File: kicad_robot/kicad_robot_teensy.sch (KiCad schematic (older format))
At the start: 2 parts, among them U12->5 R-78E5.0-1.0

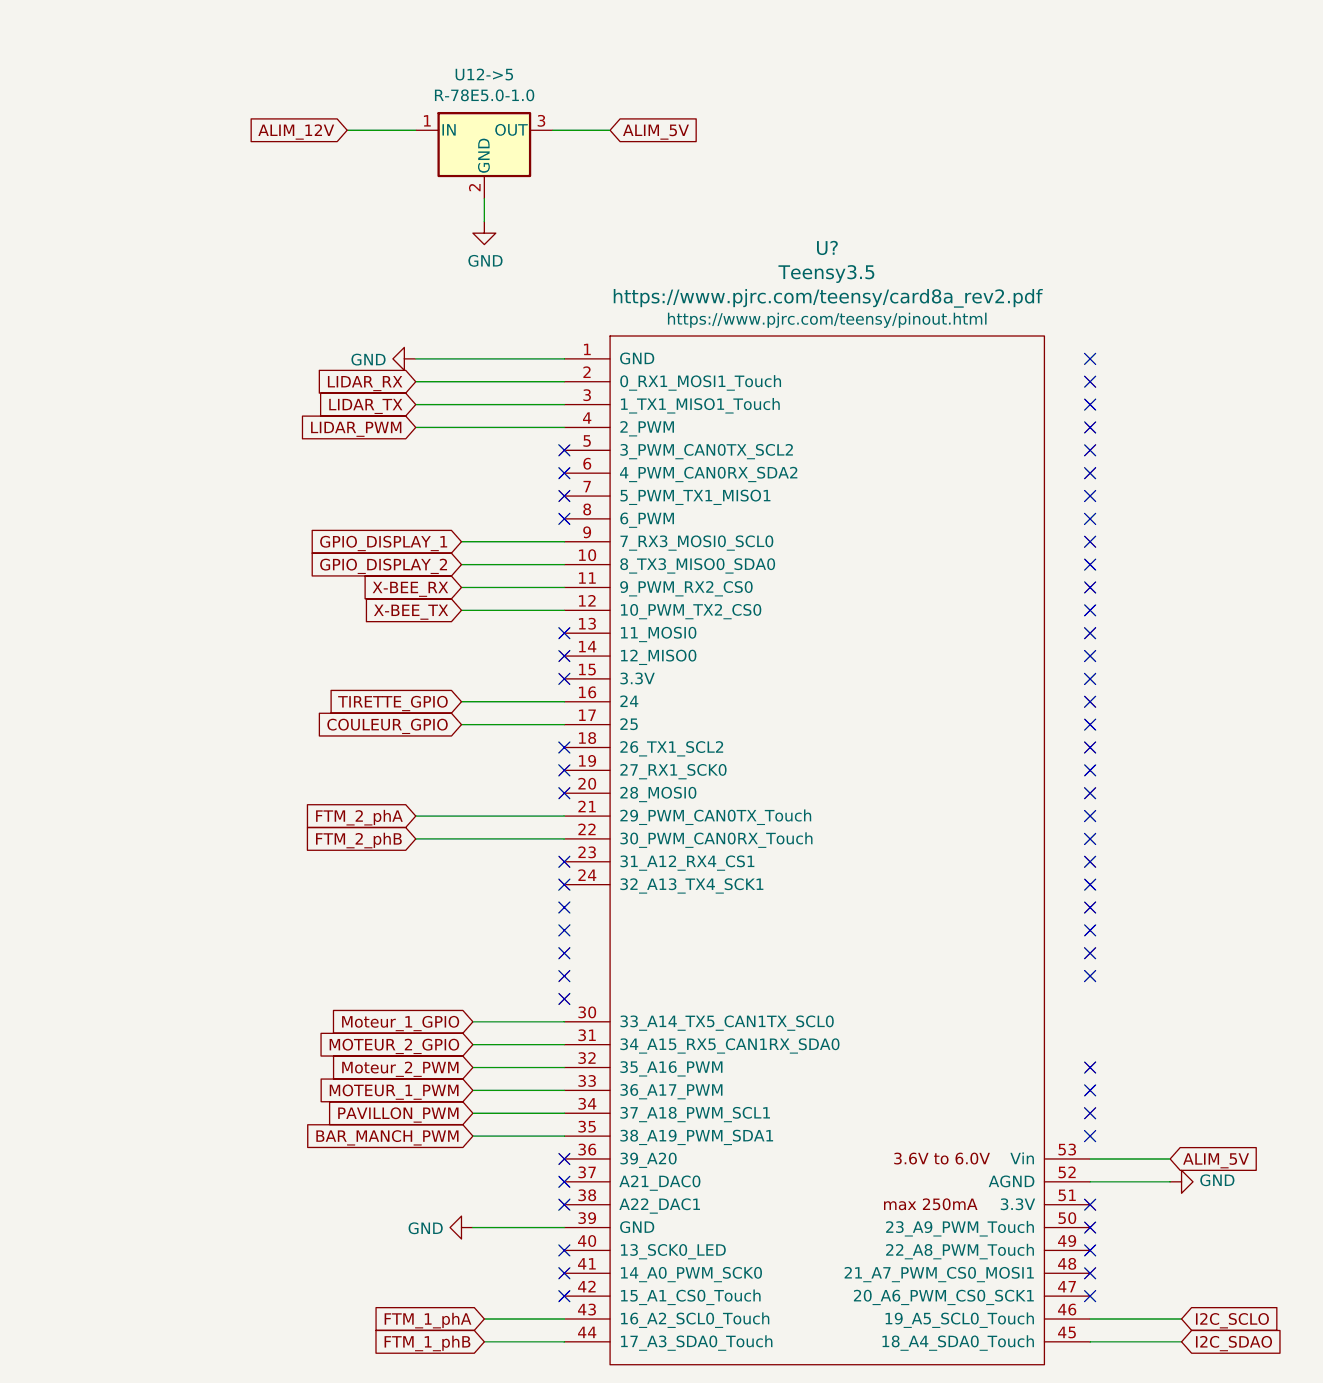
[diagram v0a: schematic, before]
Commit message: mise à jour
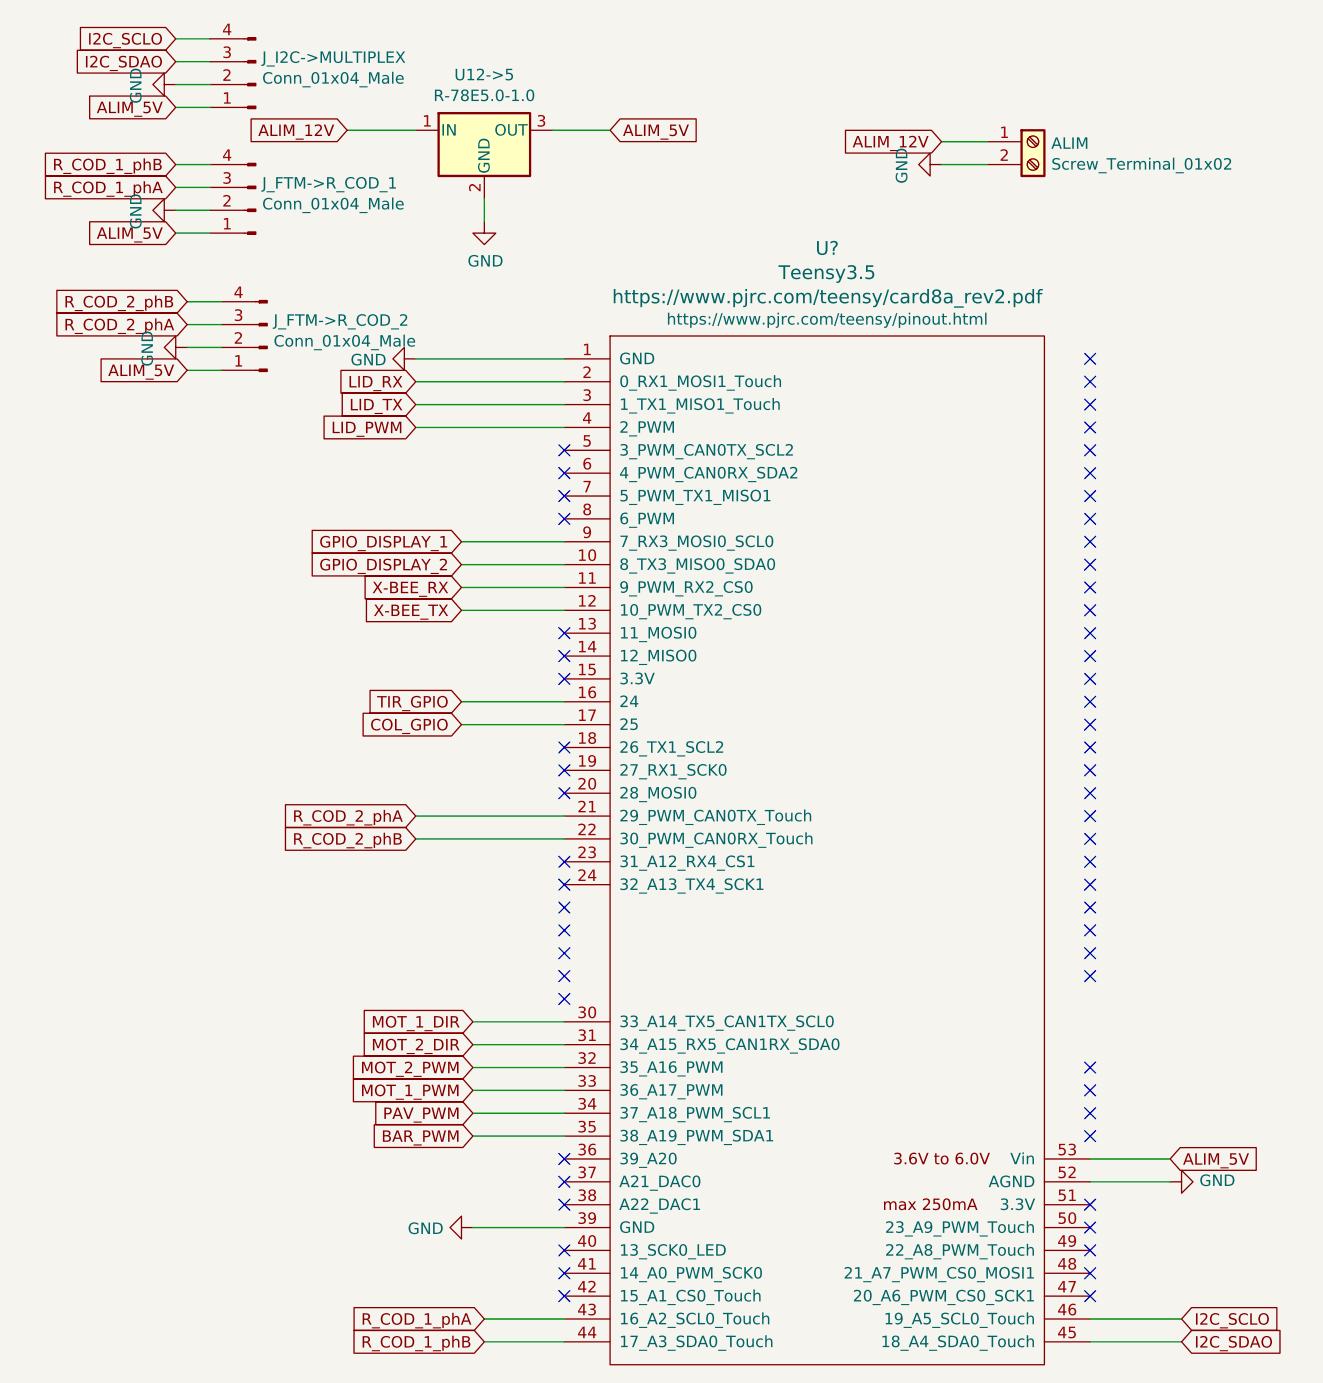
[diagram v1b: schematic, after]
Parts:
- added ALIM: Screw_Terminal_01x02, symbol Connector:Screw_Terminal_01x02
- added J_FTM->R_COD_1, J_FTM->R_COD_2, J_I2C->MULTIPLEX: Conn_01x04_Male, symbol Connector:Conn_01x04_Male
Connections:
- net ALIM_12V: now also ALIM.1 (Pin_1)
- net ALIM_5V: now also J_FTM->R_COD_1.1 (Pin_1), J_FTM->R_COD_2.1 (Pin_1), J_I2C->MULTIPLEX.1 (Pin_1)
- net GND: now also ALIM.2 (Pin_2), J_FTM->R_COD_1.2 (Pin_2), J_FTM->R_COD_2.2 (Pin_2), J_I2C->MULTIPLEX.2 (Pin_2)
- net I2C_SCLO: now also J_I2C->MULTIPLEX.4 (Pin_4)
- net I2C_SDAO: now also J_I2C->MULTIPLEX.3 (Pin_3)
- net BAR_MANCH_PWM renamed BAR_PWM
- net COULEUR_GPIO renamed COL_GPIO
- net FTM_1_phA renamed R_COD_1_phA
- net R_COD_1_phA: now also J_FTM->R_COD_1.3 (Pin_3)
- net FTM_1_phB renamed R_COD_1_phB
- net R_COD_1_phB: now also J_FTM->R_COD_1.4 (Pin_4)
- net FTM_2_phA renamed R_COD_2_phA
- net R_COD_2_phA: now also J_FTM->R_COD_2.3 (Pin_3)
- net FTM_2_phB renamed R_COD_2_phB
- net R_COD_2_phB: now also J_FTM->R_COD_2.4 (Pin_4)
- net LIDAR_PWM renamed LID_PWM
- net LIDAR_RX renamed LID_RX
- net LIDAR_TX renamed LID_TX
- net MOTEUR_1_PWM renamed MOT_1_PWM
- net MOTEUR_2_GPIO renamed MOT_2_DIR
- net Moteur_1_GPIO renamed MOT_1_DIR
- net Moteur_2_PWM renamed MOT_2_PWM
- net PAVILLON_PWM renamed PAV_PWM
- net TIRETTE_GPIO renamed TIR_GPIO
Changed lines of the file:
@@
 $EndComp
 Text GLabel 7450 2100 0    50   Input ~ 0
-LIDAR_RX
+LID_RX
 Text GLabel 7450 2200 0    50   Input ~ 0
-LIDAR_TX
+LID_TX
 Text GLabel 7450 2300 0    50   Input ~ 0
-LIDAR_PWM
+LID_PWM
 Text GLabel 7650 2800 0    50   Input ~ 0
 GPIO_DISPLAY_1
@@
 X-BEE_TX
 Text GLabel 7650 3500 0    50   Input ~ 0
-TIRETTE_GPIO
+TIR_GPIO
 $Comp
 L power:GND #PWR?
@@
 	10750 5500 10400 5500
 Text GLabel 7650 3600 0    50   Input ~ 0
-COULEUR_GPIO
+COL_GPIO
 Text GLabel 7450 4000 0    50   Input ~ 0
-FTM_2_phA
+R_COD_2_phA
 Text GLabel 7450 4100 0    50   Input ~ 0
-FTM_2_phB
+R_COD_2_phB
 Text GLabel 7700 4900 0    50   Input ~ 0
-Moteur_1_GPIO
+MOT_1_DIR
 Text GLabel 7700 5000 0    50   Input ~ 0
-MOTEUR_2_GPIO
+MOT_2_DIR
 Text GLabel 7700 5100 0    50   Input ~ 0
-Moteur_2_PWM
+MOT_2_PWM
 Text GLabel 7700 5200 0    50   Input ~ 0
-MOTEUR_1_PWM
+MOT_1_PWM
 Text GLabel 7700 5300 0    50   Input ~ 0
-PAVILLON_PWM
+PAV_PWM
 Text GLabel 7700 5400 0    50   Input ~ 0
-BAR_MANCH_PWM
+BAR_PWM
 Text GLabel 7750 6200 0    50   Input ~ 0
-FTM_1_phA
+R_COD_1_phA
 Text GLabel 7750 6300 0    50   Input ~ 0
-FTM_1_phB
+R_COD_1_phB
 Wire Wire Line
 	7750 6300 8100 6300
@@
 Wire Wire Line
 	7150 1000 7450 1000
+$Comp
+L Connector:Screw_Terminal_01x02 ALIM
+U 1 1 60342002
+P 10150 1050
+F 0 "ALIM" H 10230 1042 50  0000 L CNN
+F 1 "Screw_Terminal_01x02" H 10230 951 50  0000 L CNN
+F 2 "" H 10150 1050 50  0001 C CNN
+F 3 "~" H 10150 1050 50  0001 C CNN
+	1    10150 1050
+	1    0    0    -1
+$EndComp
+Text GLabel 9750 1050 0    50   Input ~ 0
+ALIM_12V
+$Comp
+L power:GND #PWR?
+U 1 1 60342E59
+P 9750 1150
+F 0 "#PWR?" H 9750 900 50  0001 C CNN
+F 1 "GND" H 9755 977 50  0000 C CNN
+F 2 "" H 9750 1150 50  0001 C CNN
+F 3 "" H 9750 1150 50  0001 C CNN
+	1    9750 1150
+	0    1    1    0
+$EndComp
+Wire Wire Line
+	9750 1150 9950 1150
+Wire Wire Line
+	9750 1050 9950 1050
+$Comp
+L Connector:Conn_01x04_Male J_I2C->MULTIPLEX
+U 1 1 60344D96
+P 6750 800
+F 0 "J_I2C->MULTIPLEX" H 6722 682 50  0000 R CNN
+F 1 "Conn_01x04_Male" H 6722 773 50  0000 R CNN
+F 2 "" H 6750 800 50  0001 C CNN
+F 3 "~" H 6750 800 50  0001 C CNN
+	1    6750 800
+	-1   0    0    1
+$EndComp
+$Comp
+L power:GND #PWR?
+U 1 1 6034965D
+P 6400 800
+F 0 "#PWR?" H 6400 550 50  0001 C CNN
+F 1 "GND" H 6405 627 50  0000 C CNN
+F 2 "" H 6400 800 50  0001 C CNN
+F 3 "" H 6400 800 50  0001 C CNN
+	1    6400 800
+	0    1    1    0
+$EndComp
+Text GLabel 6400 900  0    50   Input ~ 0
+ALIM_5V
+Text GLabel 6400 700  0    50   Input ~ 0
+I2C_SDAO
+Text GLabel 6400 600  0    50   Input ~ 0
+I2C_SCLO
+Wire Wire Line
+	6400 600  6550 600
+Wire Wire Line
+	6400 700  6550 700
+Wire Wire Line
+	6400 800  6550 800
+Wire Wire Line
+	6400 900  6550 900
+$Comp
+L Connector:Conn_01x04_Male J_FTM->R_COD_1
+U 1 1 6034C8A3
+P 6750 1350
+F 0 "J_FTM->R_COD_1" H 6722 1232 50  0000 R CNN
+F 1 "Conn_01x04_Male" H 6722 1323 50  0000 R CNN
+F 2 "" H 6750 1350 50  0001 C CNN
+F 3 "~" H 6750 1350 50  0001 C CNN
+	1    6750 1350
+	-1   0    0    1
+$EndComp
+Text GLabel 6400 1450 0    50   Input ~ 0
+ALIM_5V
+$Comp
+L power:GND #PWR?
+U 1 1 6034D5A6
+P 6400 1350
+F 0 "#PWR?" H 6400 1100 50  0001 C CNN
+F 1 "GND" H 6405 1177 50  0000 C CNN
+F 2 "" H 6400 1350 50  0001 C CNN
+F 3 "" H 6400 1350 50  0001 C CNN
+	1    6400 1350
+	0    1    1    0
+$EndComp
+Text GLabel 6400 1250 0    50   Input ~ 0
+R_COD_1_phA
+Text GLabel 6400 1150 0    50   Input ~ 0
+R_COD_1_phB
+Wire Wire Line
+	6400 1150 6550 1150
+Wire Wire Line
+	6550 1250 6400 1250
+Wire Wire Line
+	6400 1350 6550 1350
+Wire Wire Line
+	6550 1450 6400 1450
+$Comp
+L Connector:Conn_01x04_Male J_FTM->R_COD_2
+U 1 1 6035325F
+P 6800 1950
+F 0 "J_FTM->R_COD_2" H 6772 1832 50  0000 R CNN
+F 1 "Conn_01x04_Male" H 6772 1923 50  0000 R CNN
+F 2 "" H 6800 1950 50  0001 C CNN
+F 3 "~" H 6800 1950 50  0001 C CNN
+	1    6800 1950
+	-1   0    0    1
+$EndComp
+Text GLabel 6450 2050 0    50   Input ~ 0
+ALIM_5V
+$Comp
+L power:GND #PWR?
+U 1 1 60353D5D
+P 6450 1950
+F 0 "#PWR?" H 6450 1700 50  0001 C CNN
+F 1 "GND" H 6455 1777 50  0000 C CNN
+F 2 "" H 6450 1950 50  0001 C CNN
+F 3 "" H 6450 1950 50  0001 C CNN
+	1    6450 1950
+	0    1    1    0
+$EndComp
+Text GLabel 6450 1850 0    50   Input ~ 0
+R_COD_2_phA
+Text GLabel 6450 1750 0    50   Input ~ 0
+R_COD_2_phB
+Wire Wire Line
+	6450 1750 6600 1750
+Wire Wire Line
+	6600 1850 6450 1850
+Wire Wire Line
+	6450 1950 6600 1950
+Wire Wire Line
+	6600 2050 6450 2050
 $EndSCHEMATC

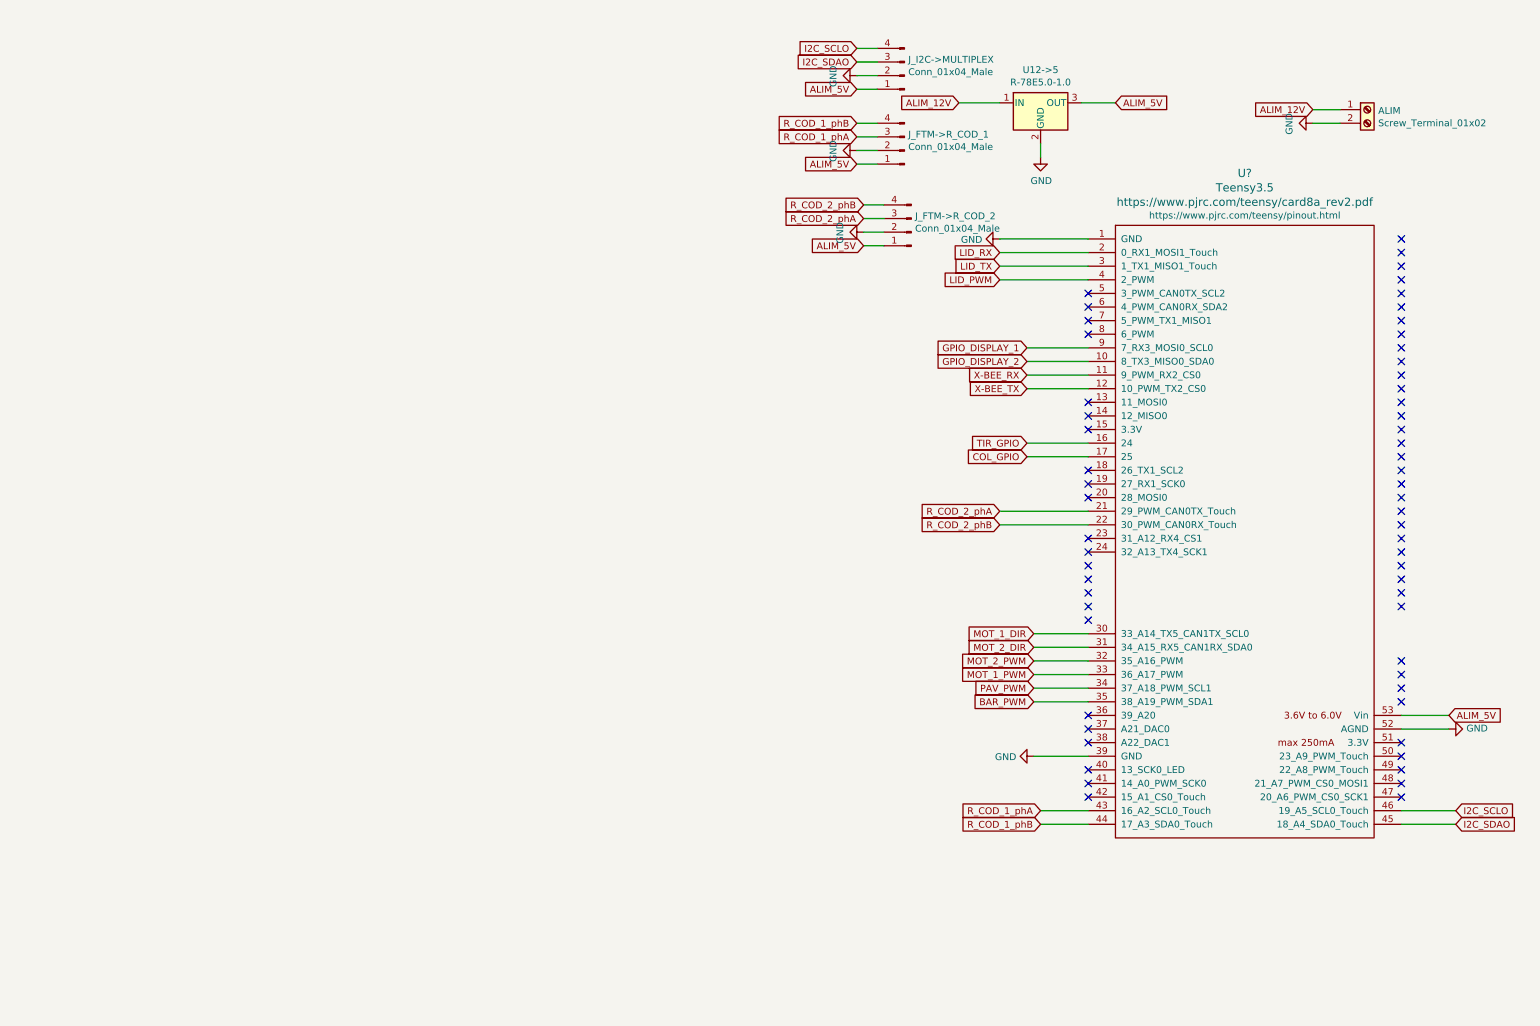
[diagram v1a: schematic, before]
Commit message: MAJ
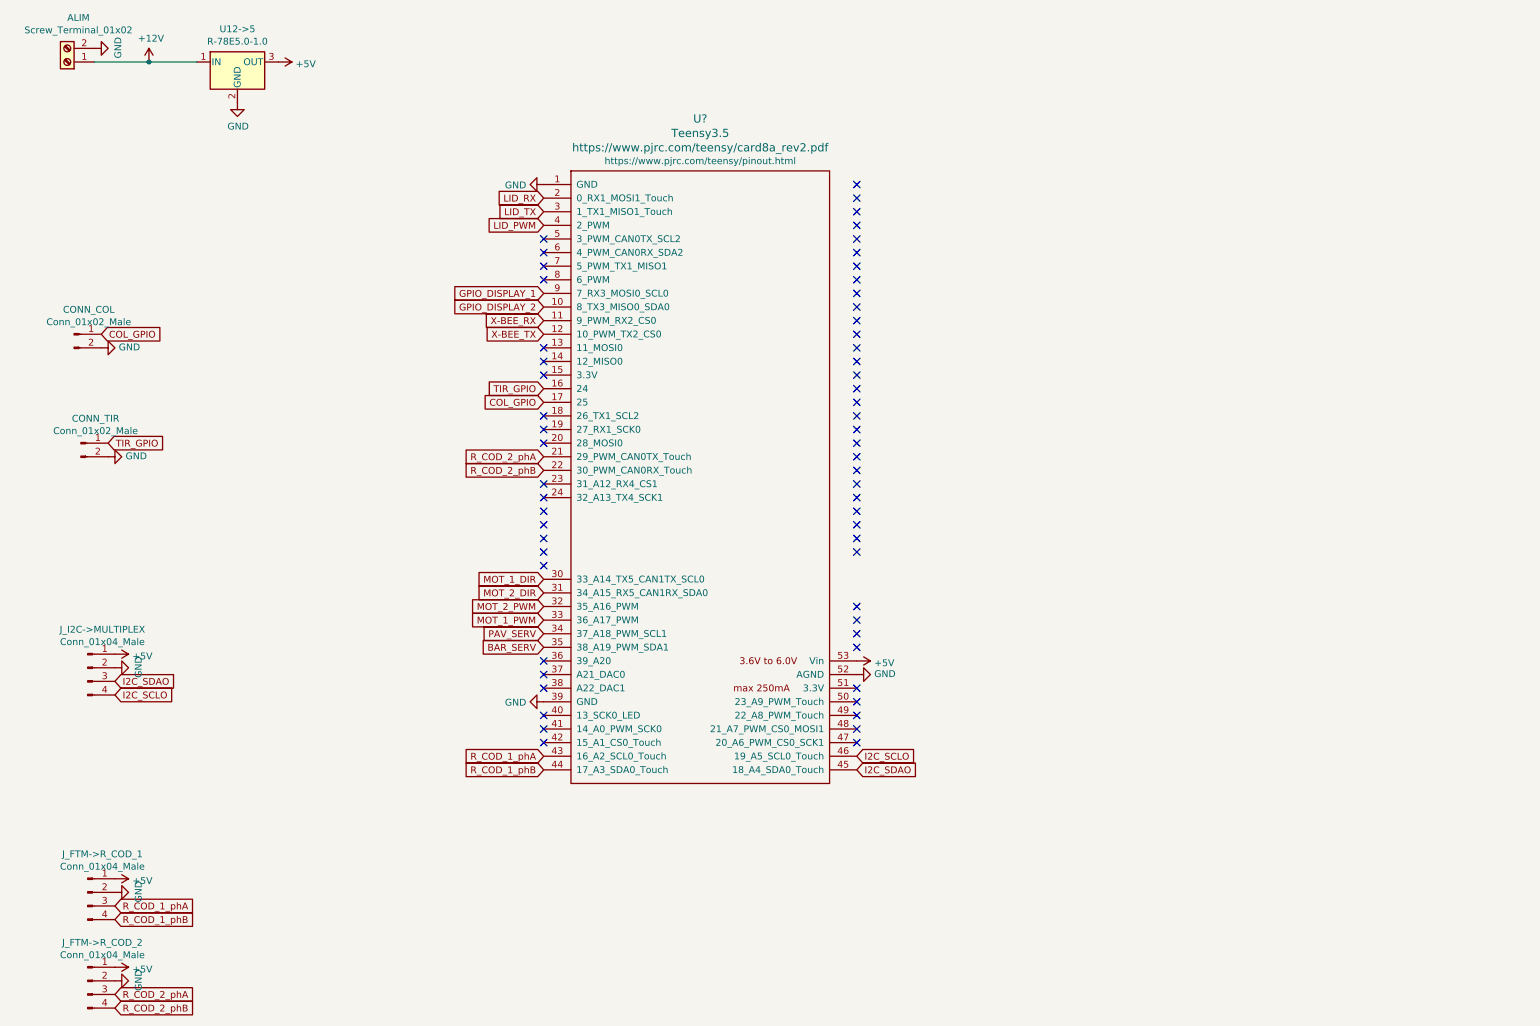
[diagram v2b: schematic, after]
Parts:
- added CONN_COL, CONN_TIR: Conn_01x02_Male, symbol Connector:Conn_01x02_Male
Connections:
- net COL_GPIO: now also CONN_COL.1 (Pin_1)
- net GND: now also CONN_COL.2 (Pin_2), CONN_TIR.2 (Pin_2)
- net TIR_GPIO: now also CONN_TIR.1 (Pin_1)
- net ALIM_12V renamed +12V
- net ALIM_5V renamed +5V
- net BAR_PWM renamed BAR_SERV
- net PAV_PWM renamed PAV_SERV
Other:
- moved on the sheet: ALIM, J_FTM->R_COD_1, J_FTM->R_COD_2, J_I2C->MULTIPLEX, U12->5, U?
